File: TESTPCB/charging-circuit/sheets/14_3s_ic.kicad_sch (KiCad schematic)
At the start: 40 parts, among them P11 1.27mm/1*3p, Q10 AO3400A, Q11 AO3401A, Q9 AO3400A, U12 BQ24170RGYR, U16 NTC10K/0805/F

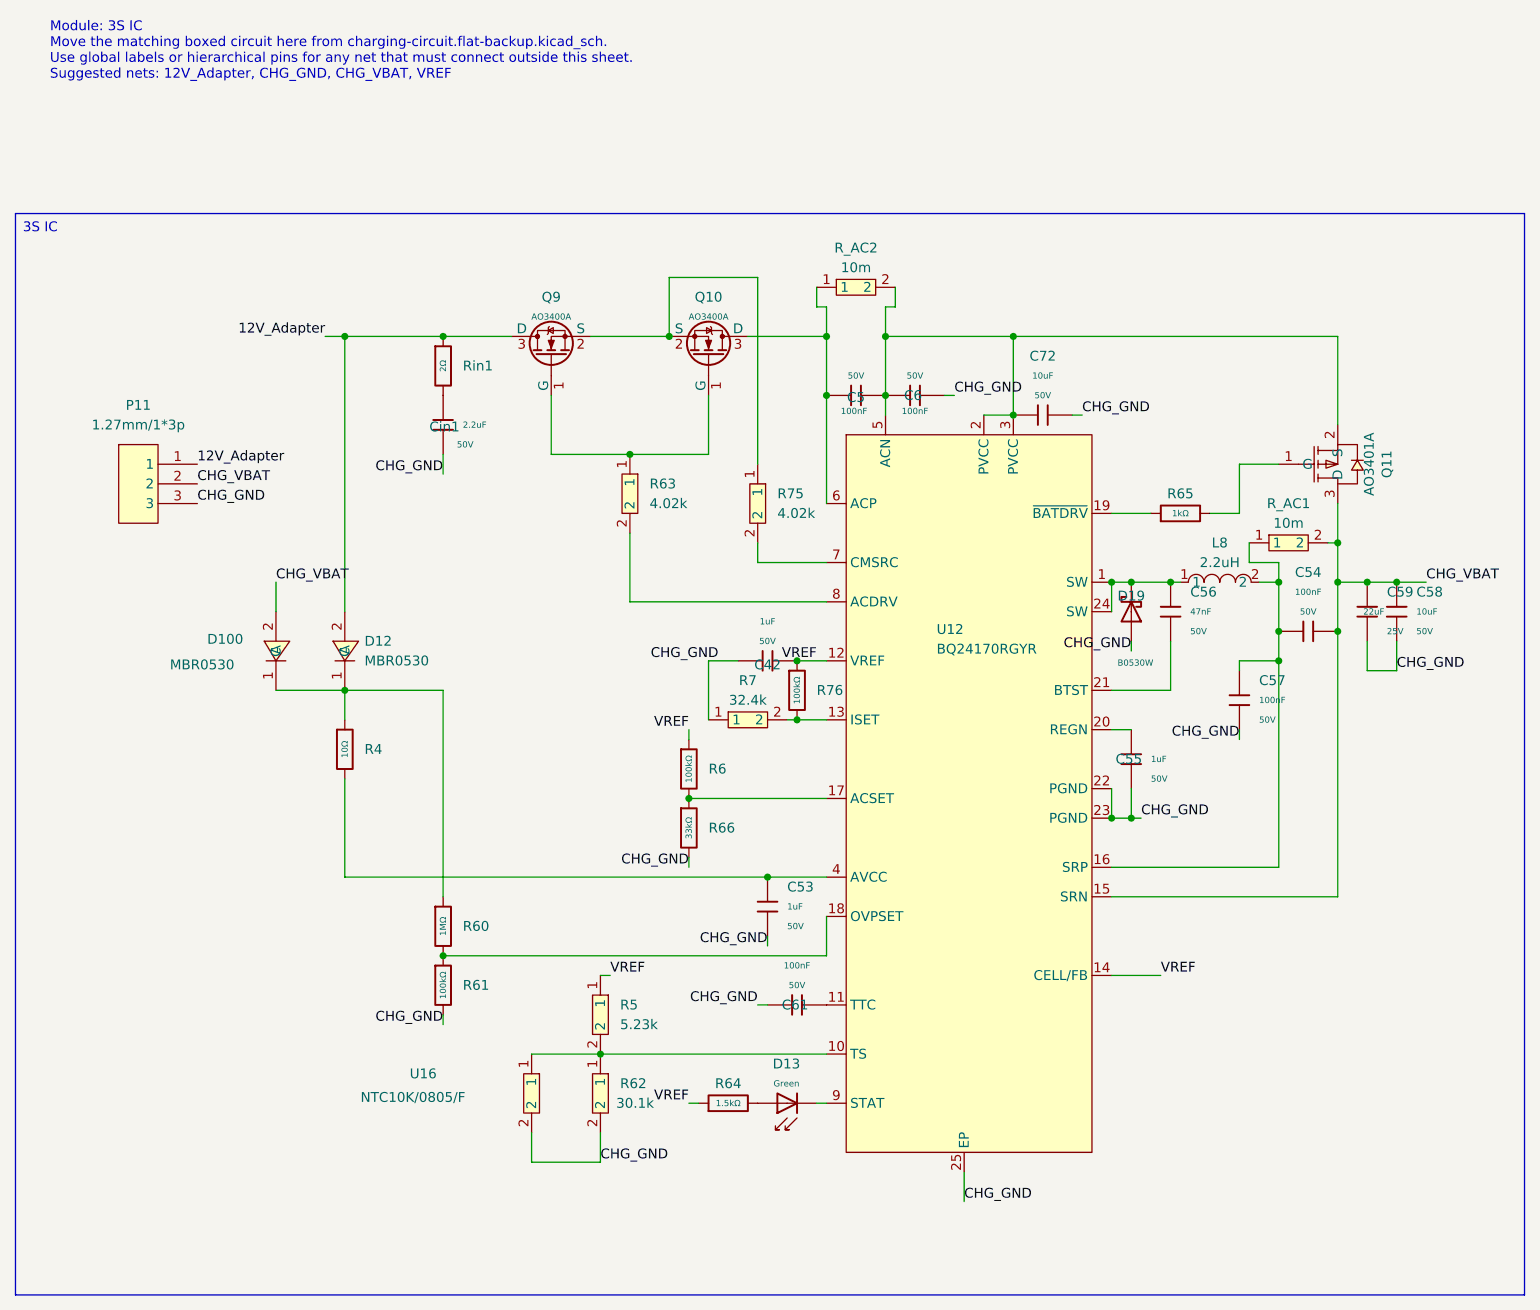
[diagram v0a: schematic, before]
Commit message: sunday
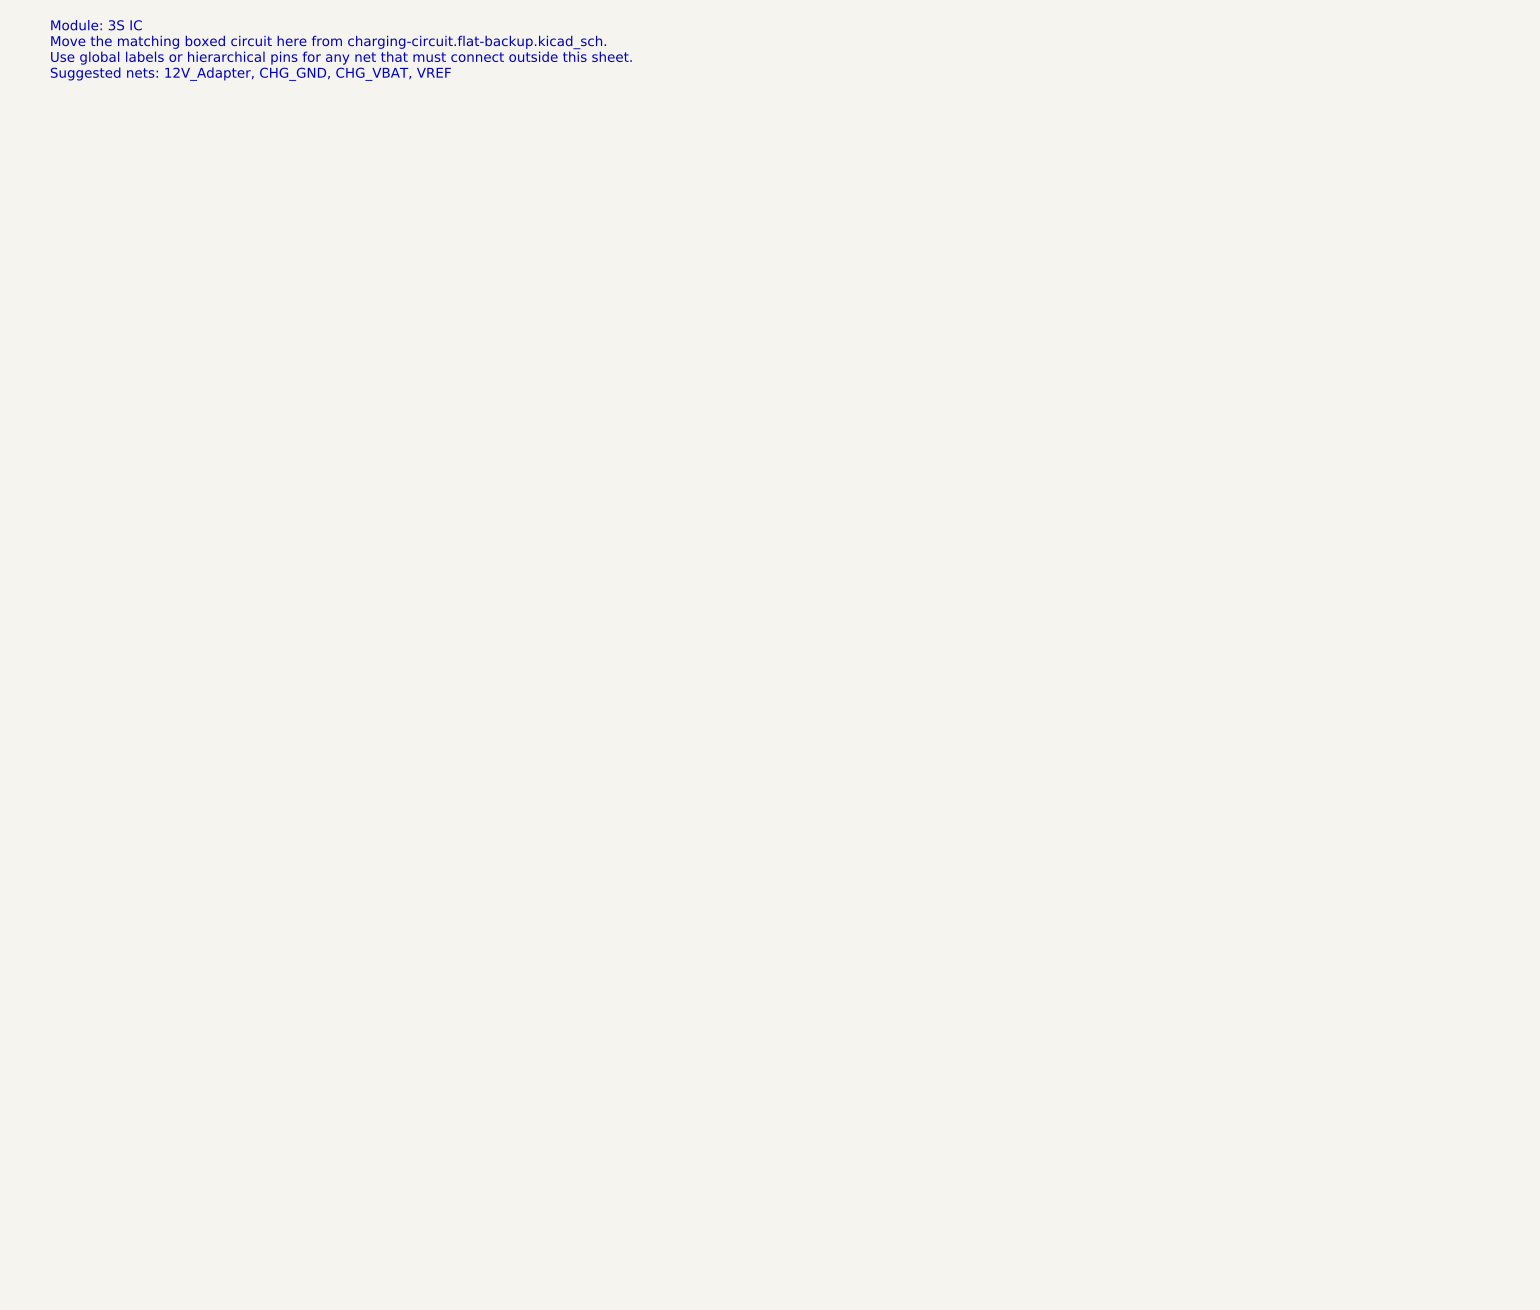
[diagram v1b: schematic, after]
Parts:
- removed C42, C53, C55: 1uF, PCM_JLCPCB:C_0603, symbol PCM_JLCPCB-Capacitors:0603,1uF
- removed C5, C54, C57, C6, C61: 100nF, PCM_JLCPCB:C_0603, symbol PCM_JLCPCB-Capacitors:0603,100nF
- removed C56: 47nF, PCM_JLCPCB:C_0603, symbol PCM_JLCPCB-Capacitors:0603,47nF
- removed C58, C72: 10uF, PCM_JLCPCB:C_1206, symbol PCM_JLCPCB-Capacitors:1206,10uF
- removed C59: 22uF, PCM_JLCPCB:C_0805, symbol PCM_JLCPCB-Capacitors:0805,22uF
- removed Cin1: 2.2uF, PCM_JLCPCB:C_0805, symbol PCM_JLCPCB-Capacitors:0805,2.2uF
- removed D100, D12: MBR0530, easyeda2kicad:SOD-123_L2.8-W1.8-LS3.7-RD, symbol easyeda2kicad:MBR0530
- removed D13: Green, PCM_JLCPCB:D_0805, symbol PCM_JLCPCB-Diodes:LED,0805,Green
- removed D19: B0530W, PCM_JLCPCB:D_SOD-123, symbol PCM_JLCPCB-Diodes:Schottky,B0530W
- removed L8: 2.2uH, easyeda2kicad:IND-SMD_L6.7-W6.6, symbol easyeda2kicad:SRP7028A-2R2M
- removed P11: 1.27mm/1*3p, easyeda2kicad:HDR-TH_3P-P1.27-V-M-1, symbol easyeda2kicad:1.27mm_1*3p
- removed Q10, Q9: AO3400A, PCM_JLCPCB:Q_SOT-23, symbol PCM_JLCPCB-Transistors:NMOS,AO3400A
- removed Q11: AO3401A, easyeda2kicad:SOT-23_L2.9-W1.3-P1.90-LS2.4-BR, symbol easyeda2kicad:AO3401A
- removed R4: 10Ω, PCM_JLCPCB:R_0402, symbol PCM_JLCPCB-Resistors:0402,10Ω
- removed R5: 5.23k, easyeda2kicad:R0805, symbol easyeda2kicad:0805W8F5231T5E
- removed R6, R61, R76: 100kΩ, PCM_JLCPCB:R_0603, symbol PCM_JLCPCB-Resistors:0603,100kΩ
- removed R60: 1MΩ, PCM_JLCPCB:R_0603, symbol PCM_JLCPCB-Resistors:0603,1MΩ
- removed R62: 30.1k, easyeda2kicad:R0603, symbol easyeda2kicad:0603WAF3012T5E
- removed R63, R75: 4.02k, easyeda2kicad:R0603, symbol easyeda2kicad:0603WAF4021T5E
- removed R64: 1.5kΩ, PCM_JLCPCB:R_0402, symbol PCM_JLCPCB-Resistors:0402,1.5kΩ
- removed R65: 1kΩ, PCM_JLCPCB:R_0603, symbol PCM_JLCPCB-Resistors:0603,1kΩ
- removed R66: 33kΩ, PCM_JLCPCB:R_0402, symbol PCM_JLCPCB-Resistors:0402,33kΩ
- removed R7: 32.4k, easyeda2kicad:R0603, symbol easyeda2kicad:0603WAF3242T5E
- removed R_AC1, R_AC2: 10m, easyeda2kicad:R1206, symbol easyeda2kicad:FMF06FTHR010-LHL
- removed Rin1: 2Ω, PCM_JLCPCB:R_0603, symbol PCM_JLCPCB-Resistors:0603,2Ω
- removed U12: BQ24170RGYR, easyeda2kicad:VQFN-24_L5.5-W3.5-P0.50-BL-EP-2, symbol easyeda2kicad:BQ24170RGYR
- removed U16: NTC10K/0805/F, easyeda2kicad:R0805, symbol easyeda2kicad:NTC10K_0805_F
